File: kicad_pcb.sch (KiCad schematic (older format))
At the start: 160 parts, among them J1 USB_B_Mini, SW1 SW_Push, U1 ATmega32U4-AU, Y1 Resonator_Small

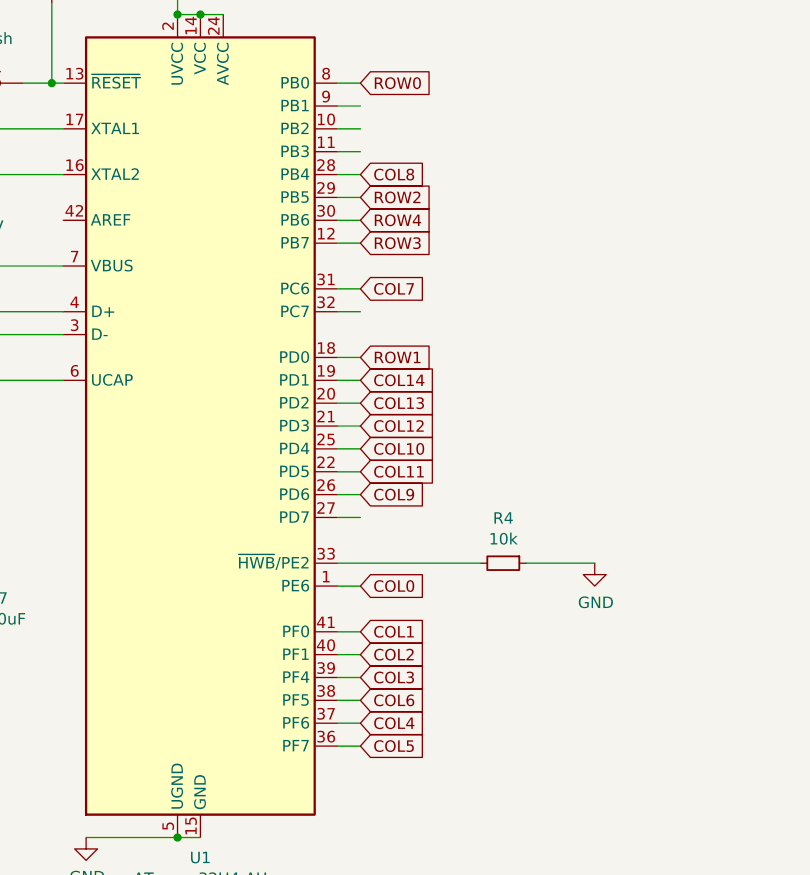
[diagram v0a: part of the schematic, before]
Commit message: further routing
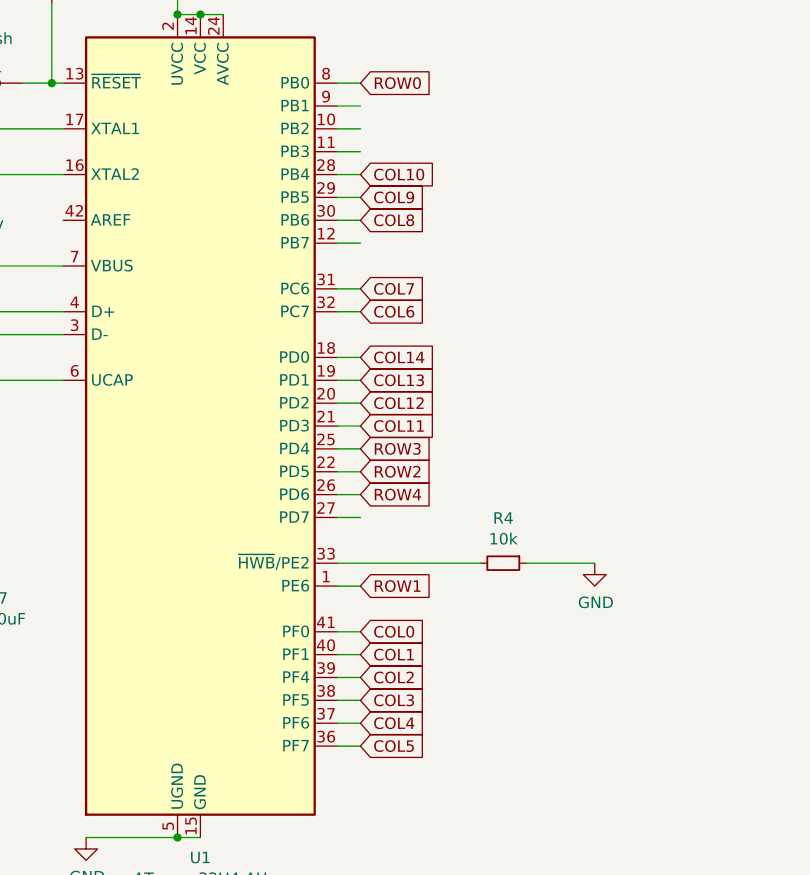
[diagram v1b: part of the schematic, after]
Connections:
- net COL0: now also U1.41 (PF0); no longer U1.1 (PE6)
- net COL1: now also U1.40 (PF1); no longer U1.41 (PF0)
- net COL10: now also U1.28 (PB4); no longer U1.25 (PD4)
- net COL11: now also U1.21 (PD3); no longer U1.22 (PD5)
- net COL12: now also U1.20 (PD2); no longer U1.21 (PD3)
- net COL13: now also U1.19 (PD1); no longer U1.20 (PD2)
- net COL14: now also U1.18 (PD0); no longer U1.19 (PD1)
- net COL2: now also U1.39 (PF4); no longer U1.40 (PF1)
- net COL3: now also U1.38 (PF5); no longer U1.39 (PF4)
- net COL6: now also U1.32 (PC7); no longer U1.38 (PF5)
- net COL8: now also U1.30 (PB6); no longer U1.28 (PB4)
- net COL9: now also U1.29 (PB5); no longer U1.26 (PD6)
- net ROW1: now also U1.1 (PE6); no longer U1.18 (PD0)
- net ROW2: now also U1.22 (PD5); no longer U1.29 (PB5)
- net ROW3: now also U1.25 (PD4); no longer U1.12 (PB7)
- net ROW4: now also U1.26 (PD6); no longer U1.30 (PB6)
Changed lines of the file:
@@
 	5000 5050 5000 6050
 Connection ~ 5000 5050
-Text GLabel 9475 10800 2    50   Input ~ 0
+Text GLabel 9475 12000 2    50   Input ~ 0
 ROW2
 Text GLabel 9475 10300 2    50   Input ~ 0
 ROW0
-Text GLabel 9475 11800 2    50   Input ~ 0
+Text GLabel 9475 11700 2    50   Input ~ 0
 COL12
-Text GLabel 9475 11700 2    50   Input ~ 0
+Text GLabel 9475 11600 2    50   Input ~ 0
 COL13
-Text GLabel 9475 11900 2    50   Input ~ 0
+Text GLabel 9475 10700 2    50   Input ~ 0
 COL10
 Text GLabel 9475 13100 2    50   Input ~ 0
@@
 Text GLabel 9475 13200 2    50   Input ~ 0
 COL5
+Text GLabel 9475 13000 2    50   Input ~ 0
+COL3
 Text GLabel 9475 12900 2    50   Input ~ 0
-COL3
-Text GLabel 9475 12500 2    50   Input ~ 0
-COL0
+COL2
 Text GLabel 9475 12800 2    50   Input ~ 0
-COL2
-Text GLabel 9475 12700 2    50   Input ~ 0
 COL1
 Connection ~ 8675 13600
@@
 	1    0    0    -1
 $EndComp
-Text GLabel 9475 11600 2    50   Input ~ 0
+Text GLabel 9475 11500 2    50   Input ~ 0
 COL14
 Wire Wire Line
@@
 Wire Wire Line
 	9475 11600 9375 11600
-Text GLabel 9475 13000 2    50   Input ~ 0
+Text GLabel 9475 11300 2    50   Input ~ 0
 COL6
-Text GLabel 9475 10700 2    50   Input ~ 0
+Text GLabel 9475 10900 2    50   Input ~ 0
 COL8
 Wire Wire Line
@@
 Wire Wire Line
 	9475 13200 9375 13200
-Text GLabel 9475 10900 2    50   Input ~ 0
+Text GLabel 9475 12100 2    50   Input ~ 0
 ROW4
-Text GLabel 9475 11000 2    50   Input ~ 0
+Text GLabel 9475 11900 2    50   Input ~ 0
 ROW3
-Text GLabel 9475 12100 2    50   Input ~ 0
+Text GLabel 9475 10800 2    50   Input ~ 0
 COL9
-Text GLabel 9475 12000 2    50   Input ~ 0
+Text GLabel 9475 11800 2    50   Input ~ 0
 COL11
 Text GLabel 9475 11200 2    50   Input ~ 0
 COL7
-Text GLabel 9475 11500 2    50   Input ~ 0
+Text GLabel 9475 12500 2    50   Input ~ 0
 ROW1
 Wire Wire Line
@@
 Wire Wire Line
 	6550 10600 6550 10650
+Text GLabel 9475 12700 2    50   Input ~ 0
+COL0
 $EndSCHEMATC
